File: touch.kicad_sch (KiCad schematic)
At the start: 12 parts, among them J3 Touch_Surface_Top, J4 Touch_Surface_Bottom, U6 CAP1208-1-A4-TR, U7 CAP1208-1-A4-TR

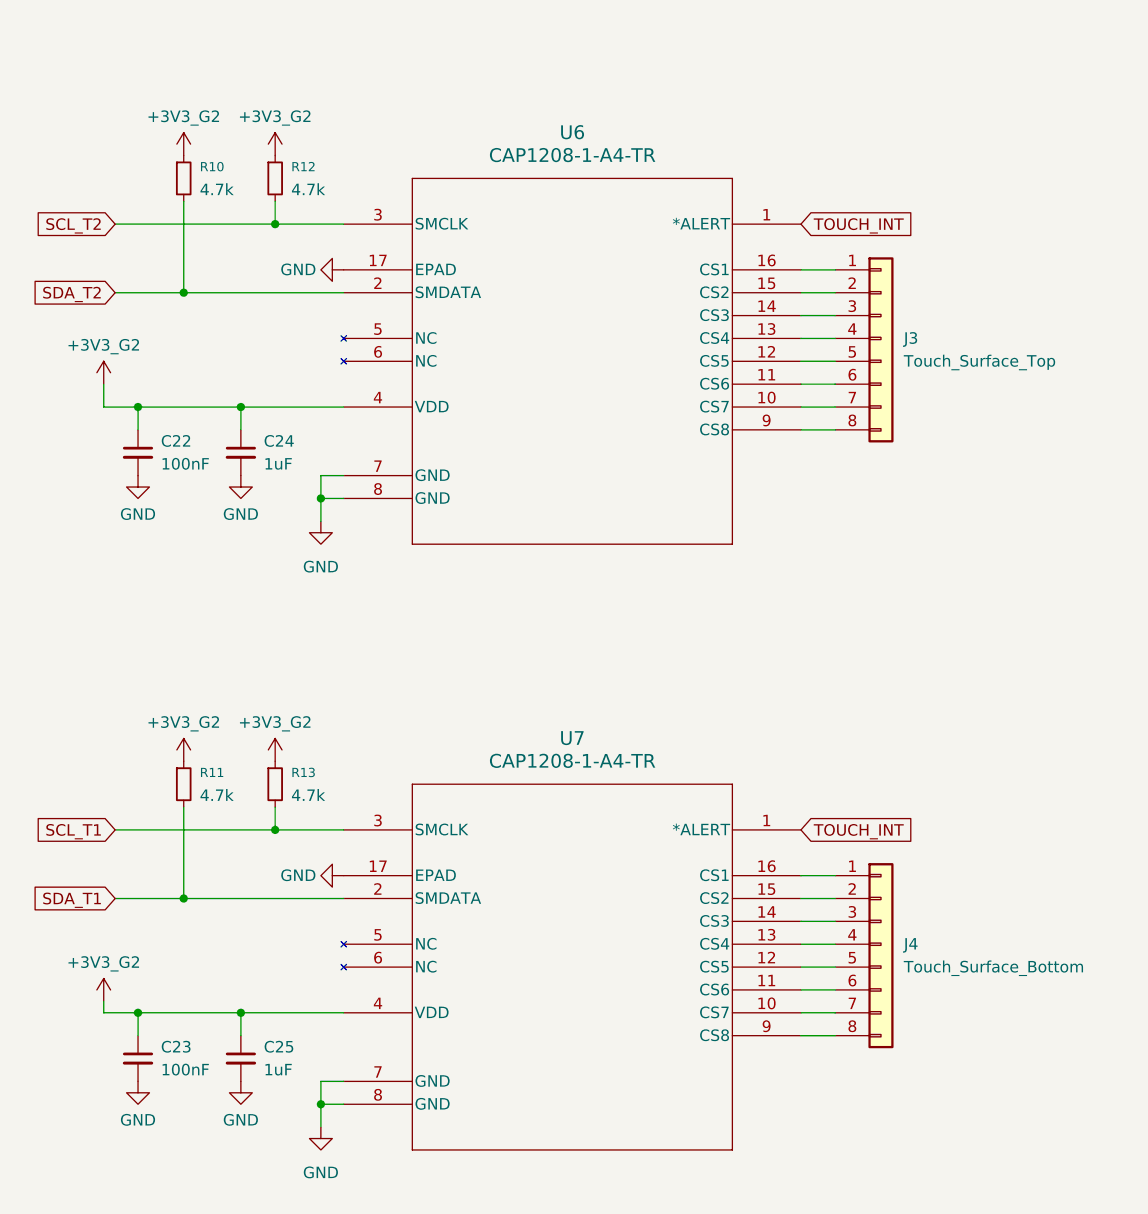
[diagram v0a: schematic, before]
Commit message: progress mid-finagling
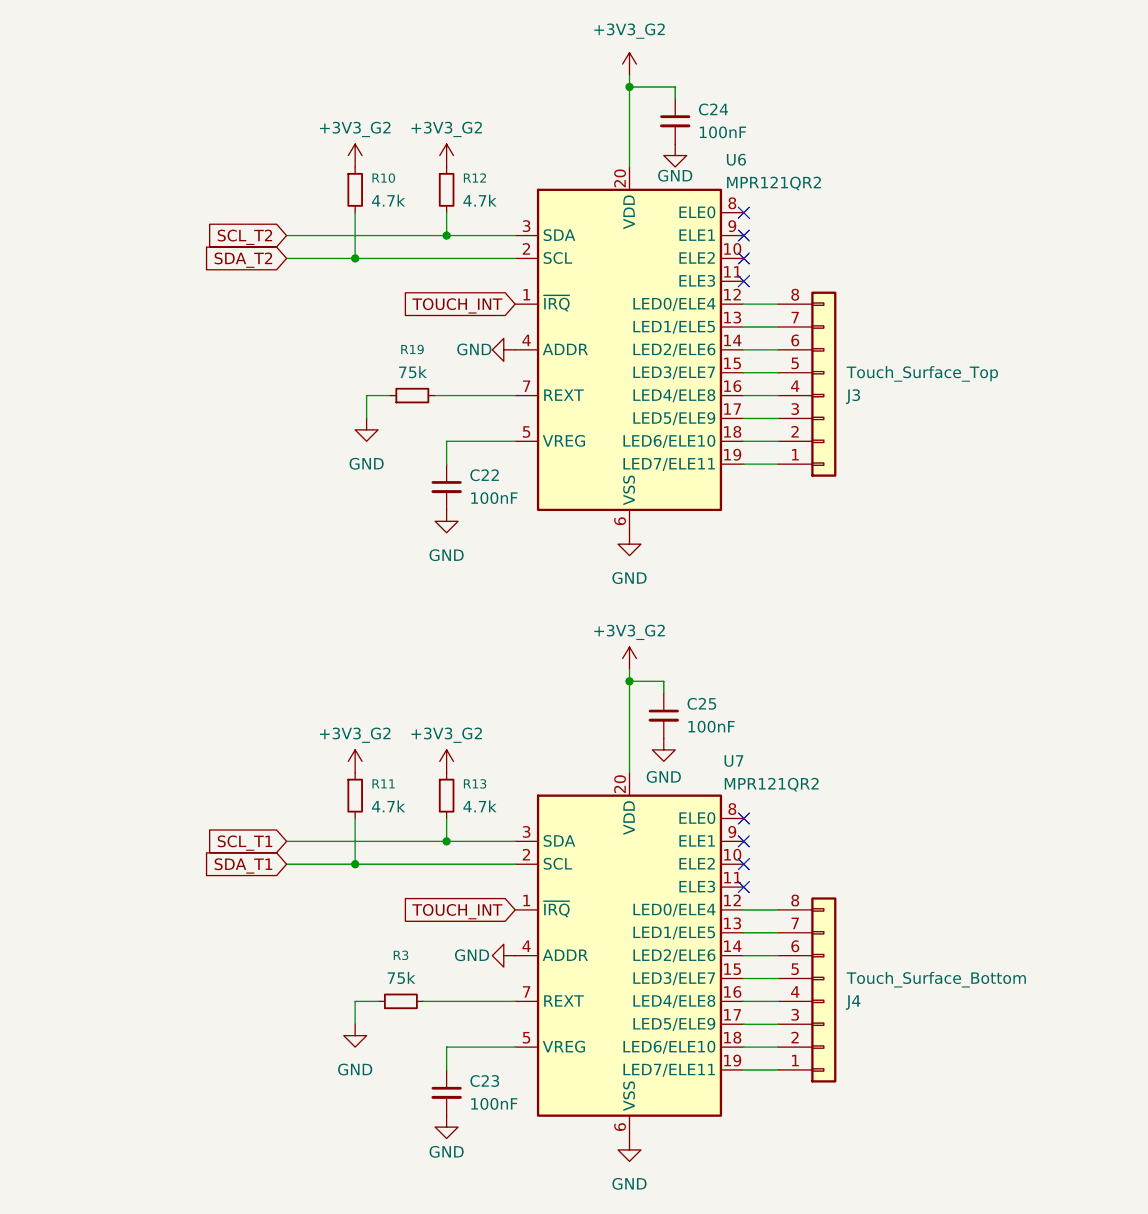
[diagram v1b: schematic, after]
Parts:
- removed U6, U7: CAP1208-1-A4-TR, QFN16_3x3MC_MCH, symbol CAP1208-1-A4-TR:CAP1208-1-A4-TR
- added R19, R3: 75k, Resistor_SMD:R_0402_1005Metric, symbol Device:R_Small
- added U6, U7: MPR121QR2, Package_DFN_QFN:UQFN-20_3x3mm_P0.4mm, symbol Sensor_Touch:MPR121QR2
- C24, C25: value 1uF -> 100nF
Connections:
- net +3V3_G2: now also U6.20 (VDD), U7.20 (VDD); no longer C22.1, C23.1
- net GND: now also R19.1, R3.1, U6.4 (ADDR), U6.6 (VSS), U7.4 (ADDR), U7.6 (VSS)
- net SCL_T1: now also U7.3 (SDA)
- net SCL_T2: now also U6.3 (SDA)
- net SDA_T1: now also U7.2 (SCL)
- net SDA_T2: now also U6.2 (SCL)
- net TOUCH_INT: now also U6.1 (~{IRQ}), U7.1 (~{IRQ})
- net at J3.1 (Pin_1): now also U6.19 (LED7/ELE11)
- net at J3.2 (Pin_2): now also U6.18 (LED6/ELE10)
- net at J3.3 (Pin_3): now also U6.17 (LED5/ELE9)
- net at J3.4 (Pin_4): now also U6.16 (LED4/ELE8)
- net at J3.5 (Pin_5): now also U6.15 (LED3/ELE7)
- net at J3.6 (Pin_6): now also U6.14 (LED2/ELE6)
- net at J3.7 (Pin_7): now also U6.13 (LED1/ELE5)
- net at J3.8 (Pin_8): now also U6.12 (LED0/ELE4)
- net at J4.7 (Pin_7): now also U7.13 (LED1/ELE5)
- net at J4.6 (Pin_6): now also U7.14 (LED2/ELE6)
- net at J4.5 (Pin_5): now also U7.15 (LED3/ELE7)
- net at J4.4 (Pin_4): now also U7.16 (LED4/ELE8)
- net at J4.3 (Pin_3): now also U7.17 (LED5/ELE9)
- net at J4.2 (Pin_2): now also U7.18 (LED6/ELE10)
- net at J4.1 (Pin_1): now also U7.19 (LED7/ELE11)
- net at J4.8 (Pin_8): now also U7.12 (LED0/ELE4)
- new net: R19.2, U6.7 (REXT)
- new net: C23.1, U7.5 (VREG)
- new net: R3.2, U7.7 (REXT)
- new net: C22.1, U6.5 (VREG)
- no-connect marks 0 -> 8
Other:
- moved on the sheet: C22, C23, C24, C25, J3, J4, R10, R11, R12, R13

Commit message: huge progress
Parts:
- U6, U7: LCSC Part (none) -> C91322
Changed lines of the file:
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@@
+			)
+		)
+		(property "LCSC Part" "C91322"
+			(at 166.37 135.89 0)
+			(effects
+				(font
+					(size 1.27 1.27)
+				)
+				(hide yes)
 			)
 		)
@@
 			(at 166.37 68.58 0)
 			(effects
+				(font
+					(size 1.27 1.27)
+				)
+				(hide yes)
+			)
+		)
+		(property "LCSC Part" "C91322"
+			(at 166.37 68.58 0)
+			(effects
